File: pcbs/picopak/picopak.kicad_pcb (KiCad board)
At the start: 4 copper layers, 50 x 21 mm, 36 parts, among them J1 USB_B_Micro, J2 Conn_02x08_Odd_Even, J3 Conn_01x03_Female, J4 Conn_01x04_Female, SW1 sw, SW2 sw, SW3 sw, SW4 sw, U1 NCP1117-3.3_SOT223, U10 74LS245, U2 W25Q128JVS, U3 RP2040, U9 74LS245, Y1 ABLS-12.000MHZ-B4-T

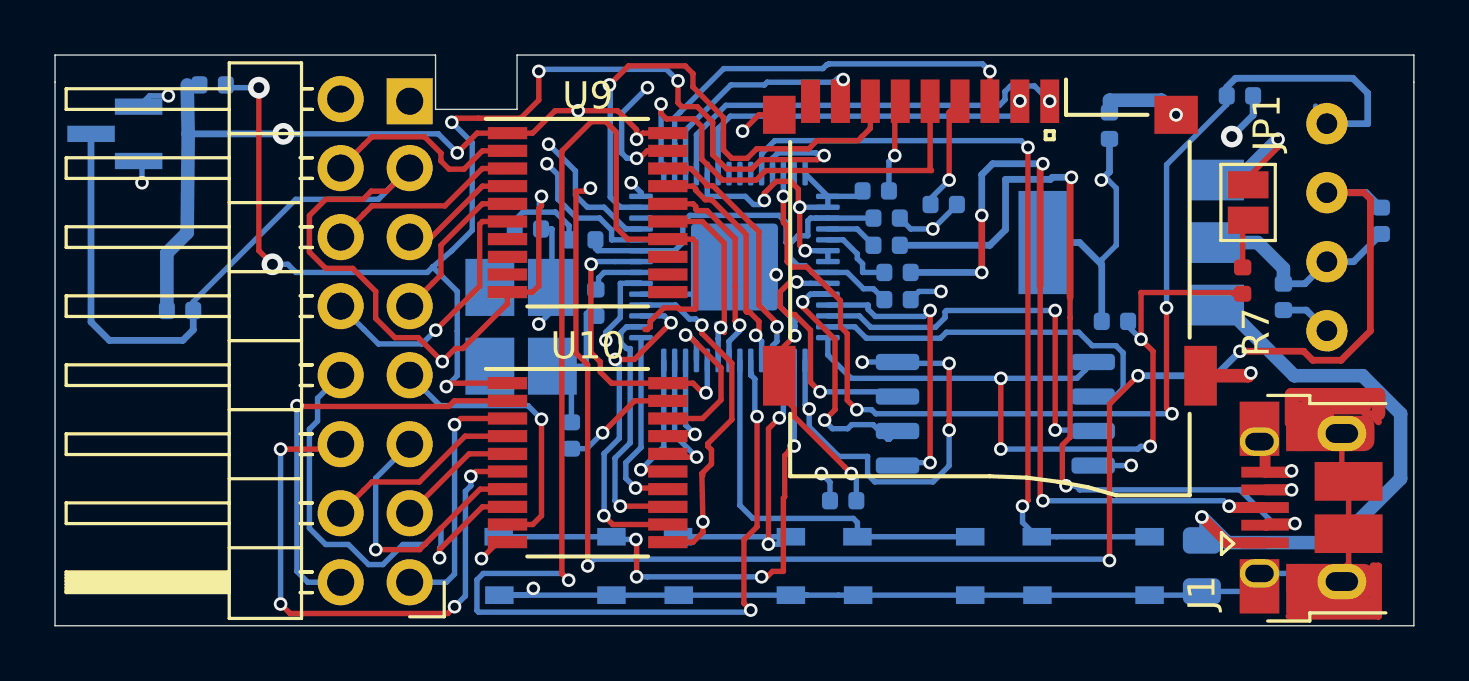
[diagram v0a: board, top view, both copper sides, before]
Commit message: V1_2 PCB laid out
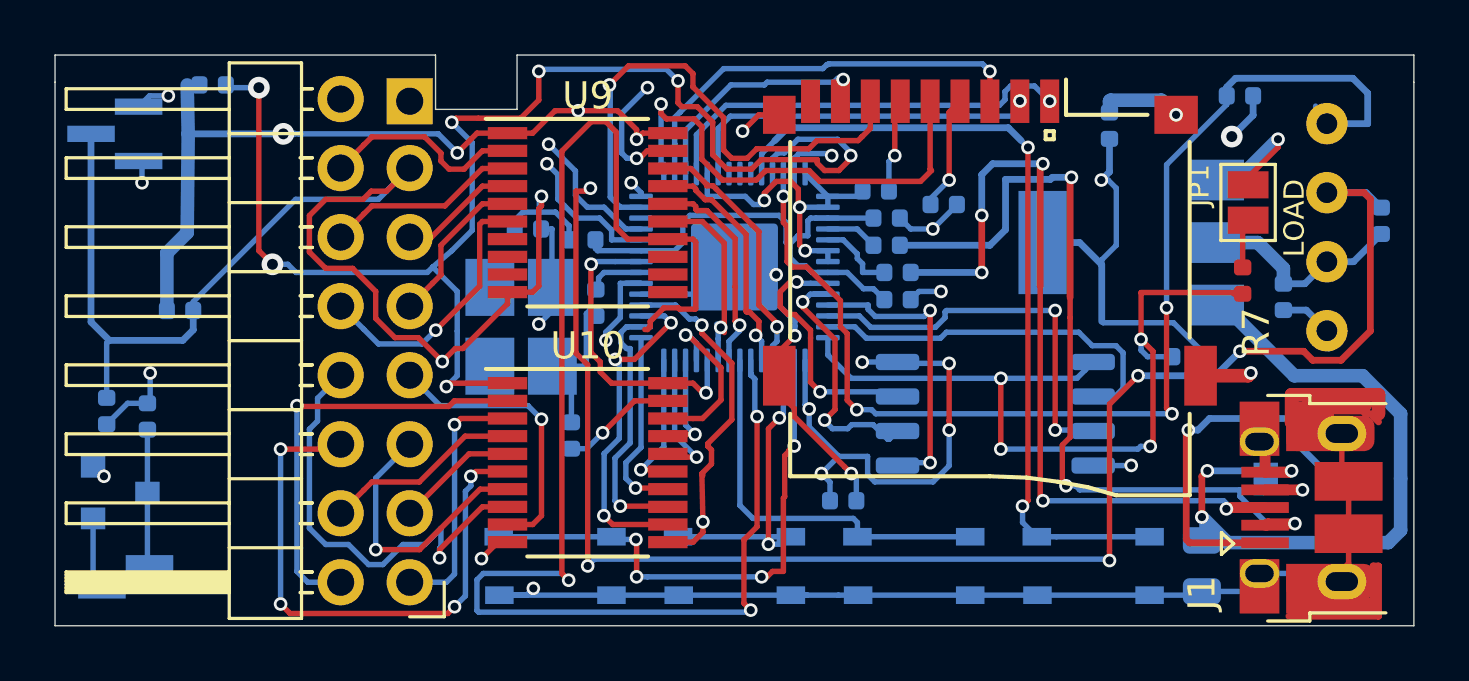
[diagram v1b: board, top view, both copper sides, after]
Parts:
- added D1: PMEG3010ER, Diode_SMD:D_SOD-123, B.Cu at (206.2, 84.6)
- added J5: Conn_01x02_Female, Connector_PinHeader_1.00mm:PinHeader_1x02_P1.00mm_Vertical_SMD_Pin1Left, B.Cu at (162.6, 88.2)
- added R8: R_Small, Capacitor_SMD:C_0402_1005Metric, B.Cu at (163.4, 82.3)
- added R9: R_Small, Capacitor_SMD:C_0402_1005Metric, B.Cu at (161.9, 82.1)
- added TR1: Si2302CDS-n-channel, Package_TO_SOT_SMD:SOT-23, B.Cu at (162.4, 85.1)
- moved R2 2.91 mm to (201.6, 80.1), turned to 180 degrees
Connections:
- C1 pad 1: VBUS -> Net-(C1-Pad1)
- J1 pad 1: VBUS -> Net-(D1-Pad2)
- U1 pad 3: VBUS -> Net-(C1-Pad1)
- U3 pad 41: (no net) -> BATSENSE
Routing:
- net Net-(C1-Pad1): track 0.00 -> 70.4 mm, vias 0 -> 3
- net BATSENSE: track 0.00 -> 33.4 mm, vias 0 -> 2
- net VBUS: track 25.7 -> 0.00 mm, vias 1 -> 0
- net Net-(D1-Pad2): track 0.00 -> 14.8 mm, vias 0 -> 1
- net +3V3: track 96.7 -> 101.9 mm
- net Net-(J5-Pad2): track 0.00 -> 4.95 mm
- net LS_DIR: track 48.4 -> 51.3 mm
- net Net-(J5-Pad1): track 0.00 -> 2.78 mm
- net GND: track 167.7 -> 169.8 mm
- net /QSPI_SS: track 29.7 -> 30.5 mm
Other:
- board text added: "LOAD"
- board text added: "VBAT"
- board text added: "VLCD"
